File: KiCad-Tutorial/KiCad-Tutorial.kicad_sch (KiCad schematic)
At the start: 10 parts, among them J1 Conn_01x20_Pin, J2 Conn_01x20_Pin, J3 USB_B_Micro, SW1 SW_MEC_5E, SW2 SW_MEC_5E, U1 TLV75801PDRV, U2 ESP32-S3-MINI-1, U3 D3V3XA4B10LP

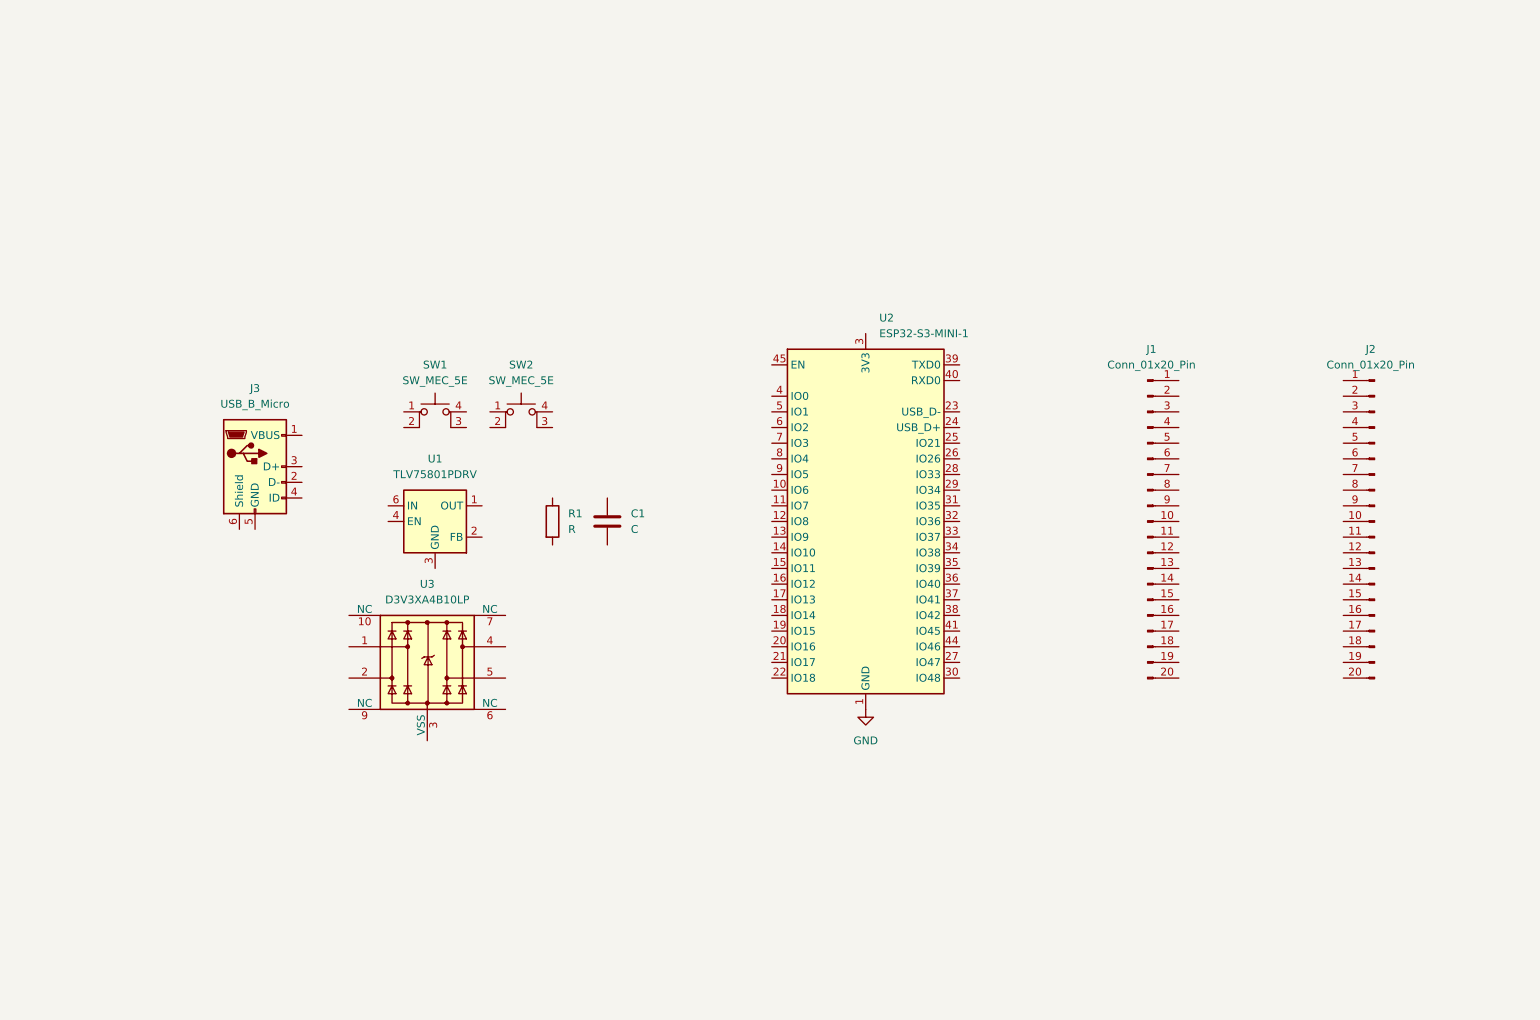
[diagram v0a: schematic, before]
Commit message: Example Done
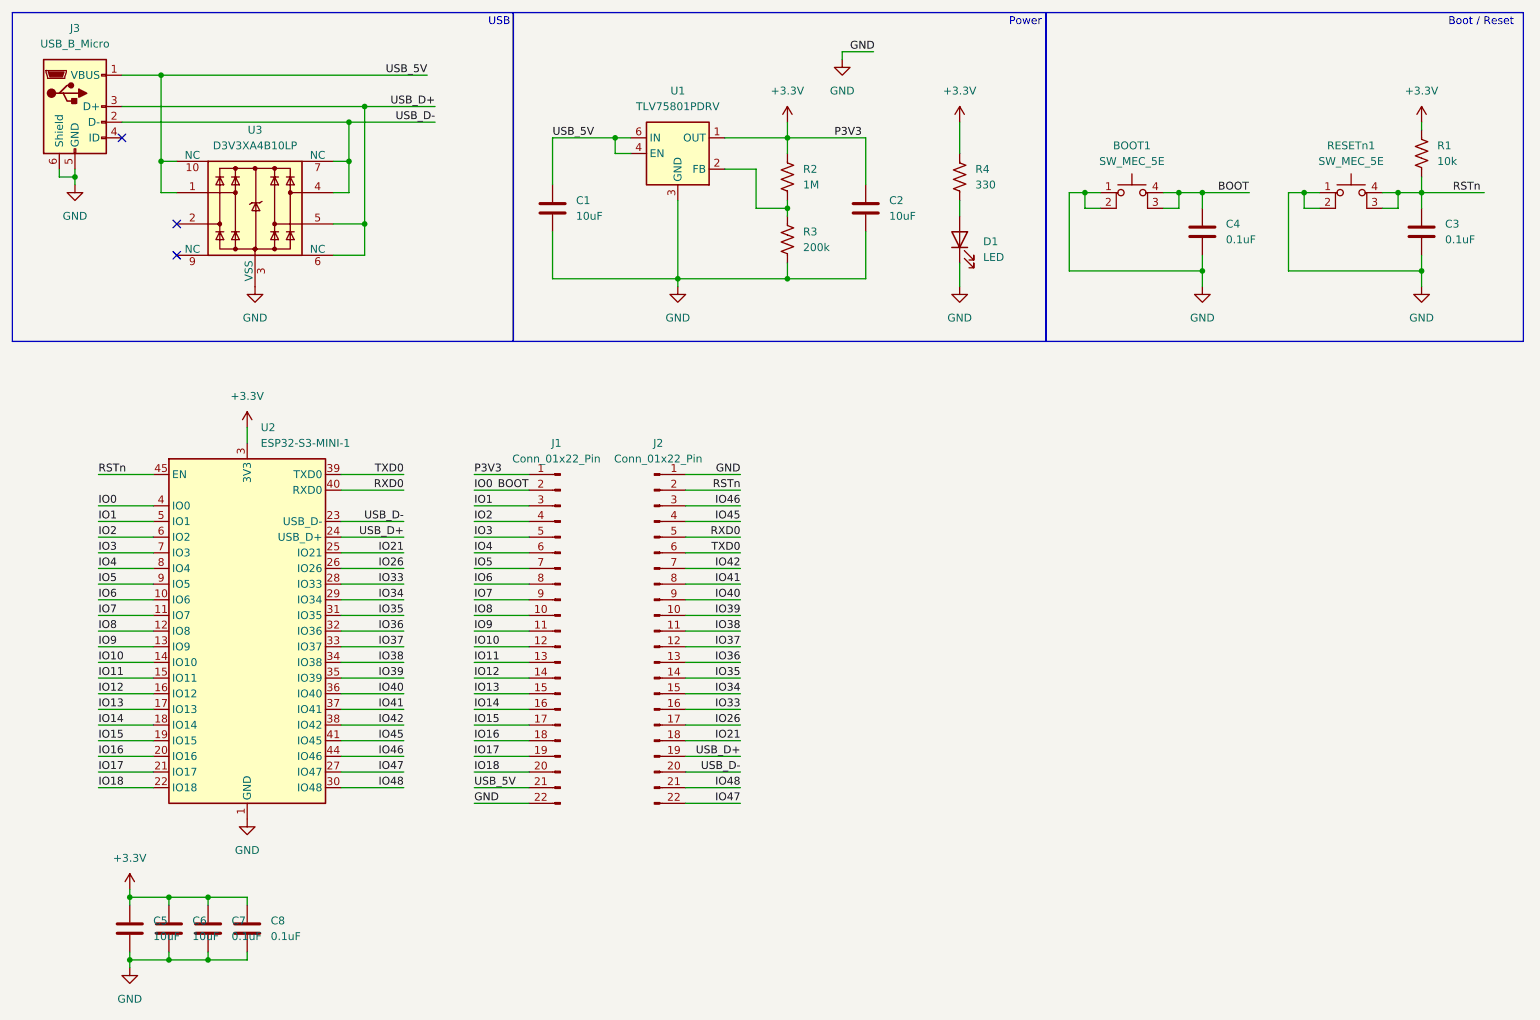
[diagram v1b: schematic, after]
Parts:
- removed J1, J2: Conn_01x20_Pin, Connector_PinHeader_2.54mm:PinHeader_1x20_P2.54mm_Vertical, symbol Connector:Conn_01x20_Pin
- removed R1: R, Resistor_SMD:R_0603_1608Metric, symbol Device:R
- added C2, C5, C6: 10uF, Capacitor_SMD:C_0603_1608Metric, symbol Device:C
- added C3, C4, C7, C8: 0.1uF, Capacitor_SMD:C_0603_1608Metric, symbol Device:C
- added D1: LED, LED_SMD:LED_0603_1608Metric, symbol Device:LED
- added J1, J2: Conn_01x22_Pin, Connector_PinHeader_2.54mm:PinHeader_1x22_P2.54mm_Vertical, symbol Connector:Conn_01x22_Pin
- added R1: 10k, Resistor_SMD:R_0603_1608Metric, symbol Device:R_US
- added R2: 1M, Resistor_SMD:R_0603_1608Metric, symbol Device:R_US
- added R3: 200k, Resistor_SMD:R_0603_1608Metric, symbol Device:R_US
- added R4: 330, Resistor_SMD:R_0603_1608Metric, symbol Device:R_US
- C1: value C -> 10uF
- renumbered SW1 to BOOT1, SW2 to RESETn1
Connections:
- net GND: now also BOOT1.1, BOOT1.2, C1.2, J3.5 (GND), J3.6 (Shield), RESETn1.1, RESETn1.2, U1.3 (GND), U1.7 (GND), U3.3 (VSS), U3.8 (VSS), C2.2, C3.2, C4.2, C5.2, C6.2, C7.2, C8.2, D1.1 (K), J1.22 (Pin_22), J2.1 (Pin_1), R3.2
- net RSTn: now reaches RESETn1.3 (K)
- net RSTn: now also RESETn1.4 (A), U2.45 (EN), C3.1, J2.2 (Pin_2), R1.2
- net USB_5V: now reaches U3.1
- net USB_5V: now also C1.1, J3.1 (VBUS), U1.4 (EN), U1.6 (IN), U3.10 (NC), J1.21 (Pin_21)
- net USB_D-: now reaches U3.4
- net USB_D-: now also J3.2 (D-), U2.23 (USB_D-), U3.7 (NC), J2.20 (Pin_20)
- net USB_D+: now reaches U3.5
- net USB_D+: now also J3.3 (D+), U2.24 (USB_D+), U3.6 (NC), J2.19 (Pin_19)
- net IO6: now reaches U2.10 (IO6)
- net IO6: now also J1.8 (Pin_8)
- net IO7: now reaches U2.11 (IO7)
- net IO7: now also J1.9 (Pin_9)
- net IO8: now reaches U2.12 (IO8)
- net IO8: now also J1.10 (Pin_10)
- net IO9: now reaches U2.13 (IO9)
- net IO9: now also J1.11 (Pin_11)
- net IO10: now reaches U2.14 (IO10)
- net IO10: now also J1.12 (Pin_12)
- net IO11: now reaches U2.15 (IO11)
- net IO11: now also J1.13 (Pin_13)
- net IO12: now reaches U2.16 (IO12)
- net IO12: now also J1.14 (Pin_14)
- net IO13: now reaches U2.17 (IO13)
- net IO13: now also J1.15 (Pin_15)
- net IO14: now reaches U2.18 (IO14)
- net IO14: now also J1.16 (Pin_16)
- net IO15: now reaches U2.19 (IO15)
- net IO15: now also J1.17 (Pin_17)
- net IO16: now reaches U2.20 (IO16)
- net IO16: now also J1.18 (Pin_18)
- net IO17: now reaches U2.21 (IO17)
- net IO17: now also J1.19 (Pin_19)
- net IO18: now reaches U2.22 (IO18)
- net IO18: now also J1.20 (Pin_20)
- net IO21: now reaches U2.25 (IO21)
- net IO21: now also J2.18 (Pin_18)
- net IO26: now reaches U2.26 (IO26)
- net IO26: now also J2.17 (Pin_17)
- net IO47: now reaches U2.27 (IO47)
- net IO47: now also J2.22 (Pin_22)
- net IO33: now reaches U2.28 (IO33)
- net IO33: now also J2.16 (Pin_16)
- net IO34: now reaches U2.29 (IO34)
- net IO34: now also J2.15 (Pin_15)
- net +3.3V: now reaches U2.3 (3V3)
- net +3.3V: now also U1.1 (OUT), C2.1, C5.1, C6.1, C7.1, C8.1, J1.1 (Pin_1), R1.1, R2.1, R4.1
- net IO48: now reaches U2.30 (IO48)
- net IO48: now also J2.21 (Pin_21)
- net IO35: now reaches U2.31 (IO35)
- net IO35: now also J2.14 (Pin_14)
- net IO36: now reaches U2.32 (IO36)
- net IO36: now also J2.13 (Pin_13)
- net IO37: now reaches U2.33 (IO37)
- net IO37: now also J2.12 (Pin_12)
- net IO38: now reaches U2.34 (IO38)
- net IO38: now also J2.11 (Pin_11)
- net IO39: now reaches U2.35 (IO39)
- net IO39: now also J2.10 (Pin_10)
- net IO40: now reaches U2.36 (IO40)
- net IO40: now also J2.9 (Pin_9)
- net IO41: now reaches U2.37 (IO41)
- net IO41: now also J2.8 (Pin_8)
- net IO42: now reaches U2.38 (IO42)
- net IO42: now also J2.7 (Pin_7)
- net TXD0: now reaches U2.39 (TXD0)
- net TXD0: now also J2.6 (Pin_6)
- net BOOT: now reaches U2.4 (IO0)
- net BOOT: now also BOOT1.3 (K), BOOT1.4 (A), C4.1, J1.2 (Pin_2)
- net RXD0: now reaches U2.40 (RXD0)
- net RXD0: now also J2.5 (Pin_5)
- net IO45: now reaches U2.41 (IO45)
- net IO45: now also J2.4 (Pin_4)
- net IO46: now reaches U2.44 (IO46)
- net IO46: now also J2.3 (Pin_3)
- net IO1: now reaches U2.5 (IO1)
- net IO1: now also J1.3 (Pin_3)
- net IO2: now reaches U2.6 (IO2)
- net IO2: now also J1.4 (Pin_4)
- net IO3: now reaches U2.7 (IO3)
- net IO3: now also J1.5 (Pin_5)
- net IO4: now reaches U2.8 (IO4)
- net IO4: now also J1.6 (Pin_6)
- net IO5: now reaches U2.9 (IO5)
- net IO5: now also J1.7 (Pin_7)
- net at U1.2 (FB): now also R2.2, R3.1
- new net: D1.2 (A), R4.2
- no-connect marks 0 -> 3
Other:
- note added: "Boot / Reset"
- note added: "Power"
- note added: "USB"
- moved on the sheet: BOOT1, C1, J3, RESETn1, U1, U2, U3
